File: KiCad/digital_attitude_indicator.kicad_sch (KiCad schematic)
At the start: 2 parts, among them U1 MPU-6050

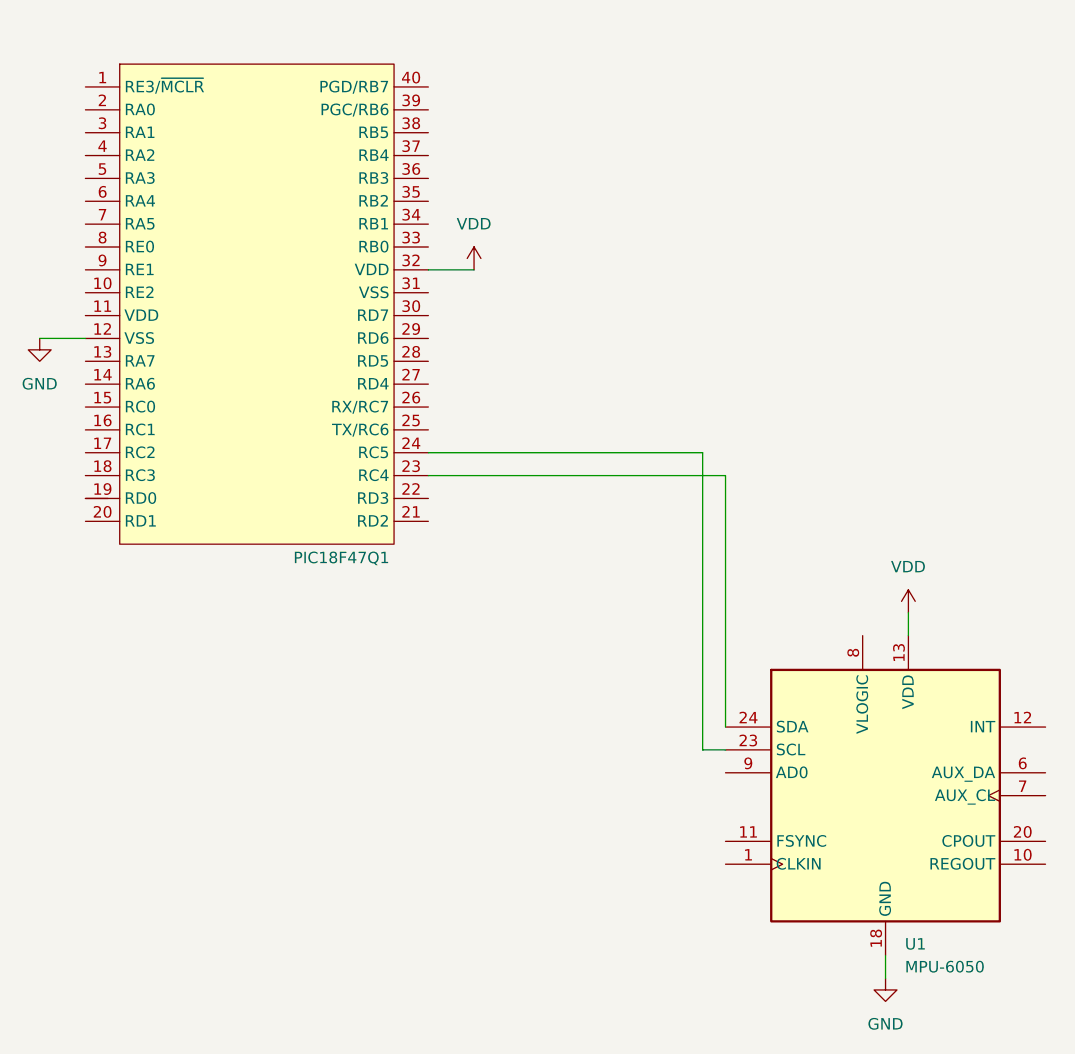
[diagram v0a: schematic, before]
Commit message: Adjuster BOM
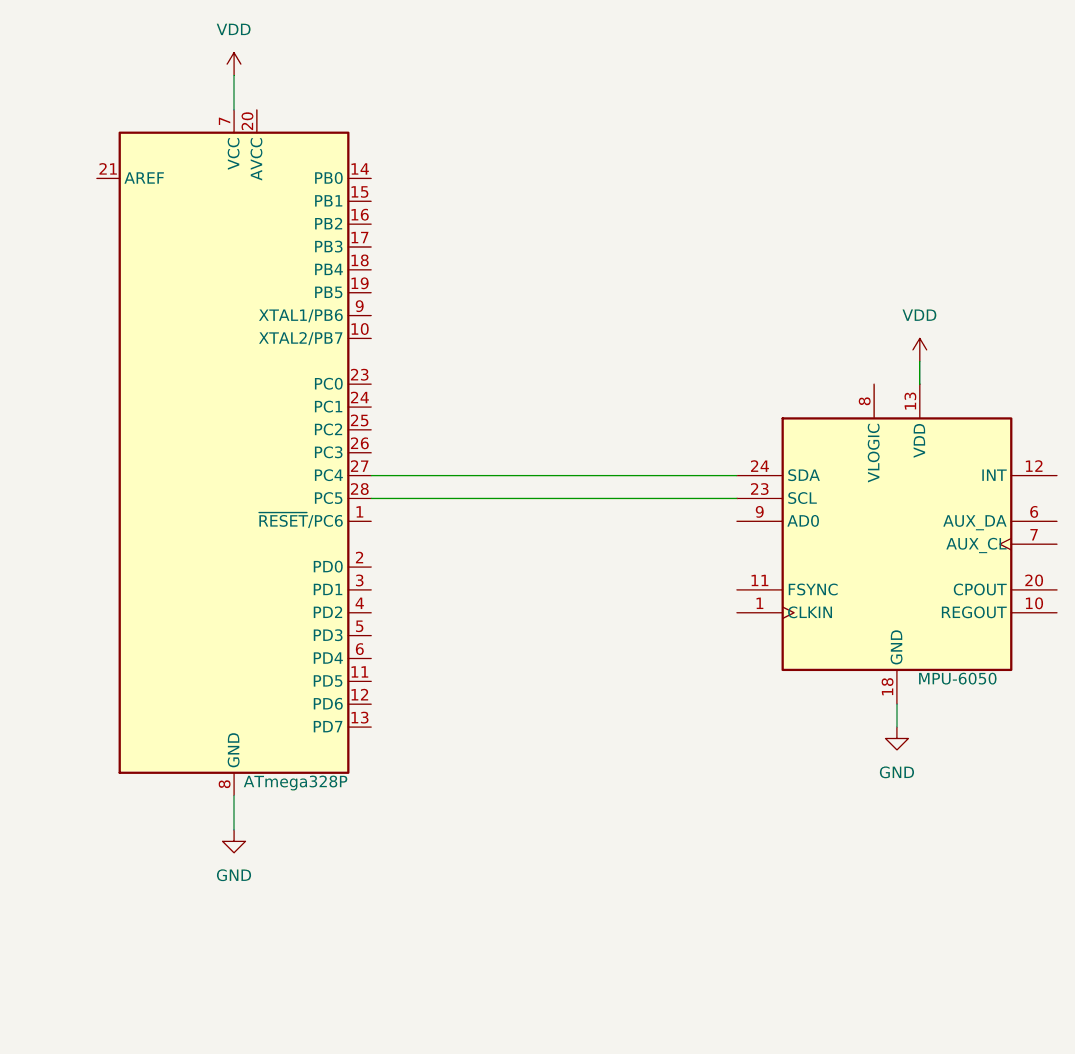
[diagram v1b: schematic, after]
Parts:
- removed PIC18F47Q1: ~, symbol MCU_Microchip_PIC18:PIC18F47Q10
- added U2: ATmega328P, Package_DIP:DIP-28_W7.62mm, symbol MCU_Microchip_ATmega:ATmega328P-P
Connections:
- net GND: now also U2.22 (GND), U2.8 (GND)
- net VDD: now also U2.7 (VCC)
- net at U1.23 (SCL): now also U2.28 (PC5)
- net at U1.24 (SDA): now also U2.27 (PC4)
